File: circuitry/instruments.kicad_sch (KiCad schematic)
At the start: 70 parts, among them J38 P9-1, J39 P9-2, J40 P7-1, J41 P7-2, J42 P8-2, J43 P8-1, J49 P10-1, J50 P10-2, J53 P1-2, J54 P2-2, J55 P3-2, J56 P4-2, J57 P17-2, J58 P18-2, J59 P12-2, J60 P11-2, J63 P14-3, J64 P13-3, J72 P16-2, J73 P15-2, J76 P16-1, J77 P15-1, J78 P16-3, J79 P15-3, J81 P19-2, J82 P17-1, J83 P18-1, J88 P5-1, J89 P6-1, J90 P5-2, J91 P6-2, J92 P6-3, J93 P5-3, M1 105ZDY08, M2 12025, M3 9733, SW1 6A Momentary, SW2 6A SPDT, SW3 6A SPDT, SW4 6A Momentary SPDT, SW5 6A SPDT

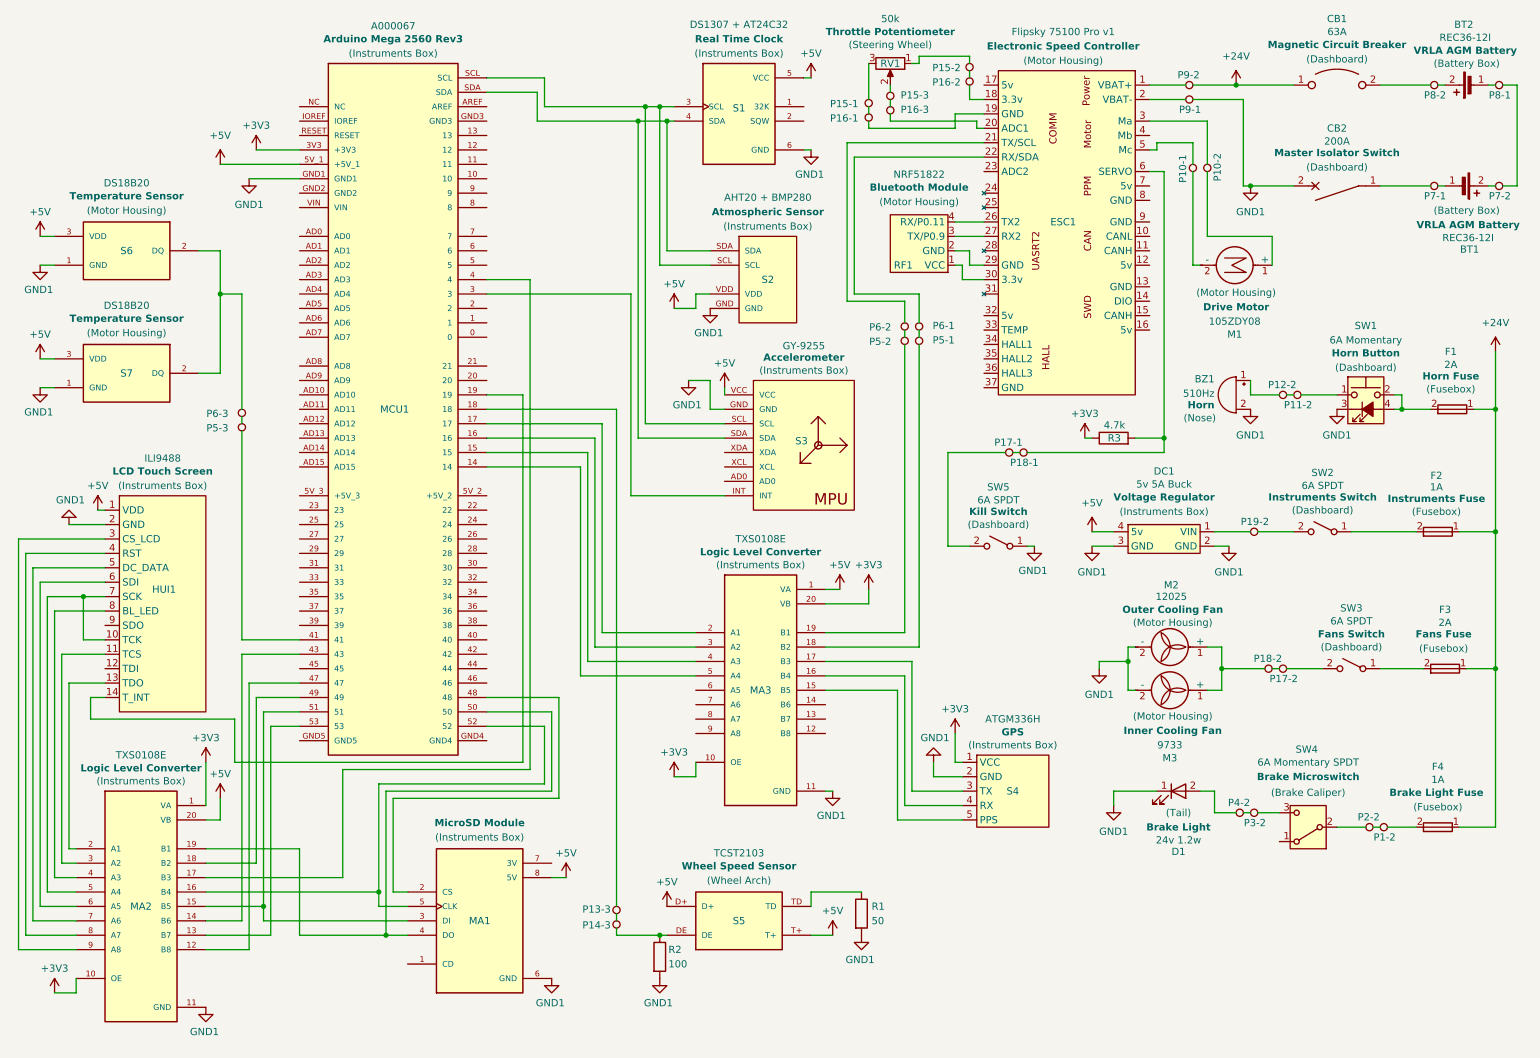
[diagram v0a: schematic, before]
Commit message: feat: Major circuit revision & refactor
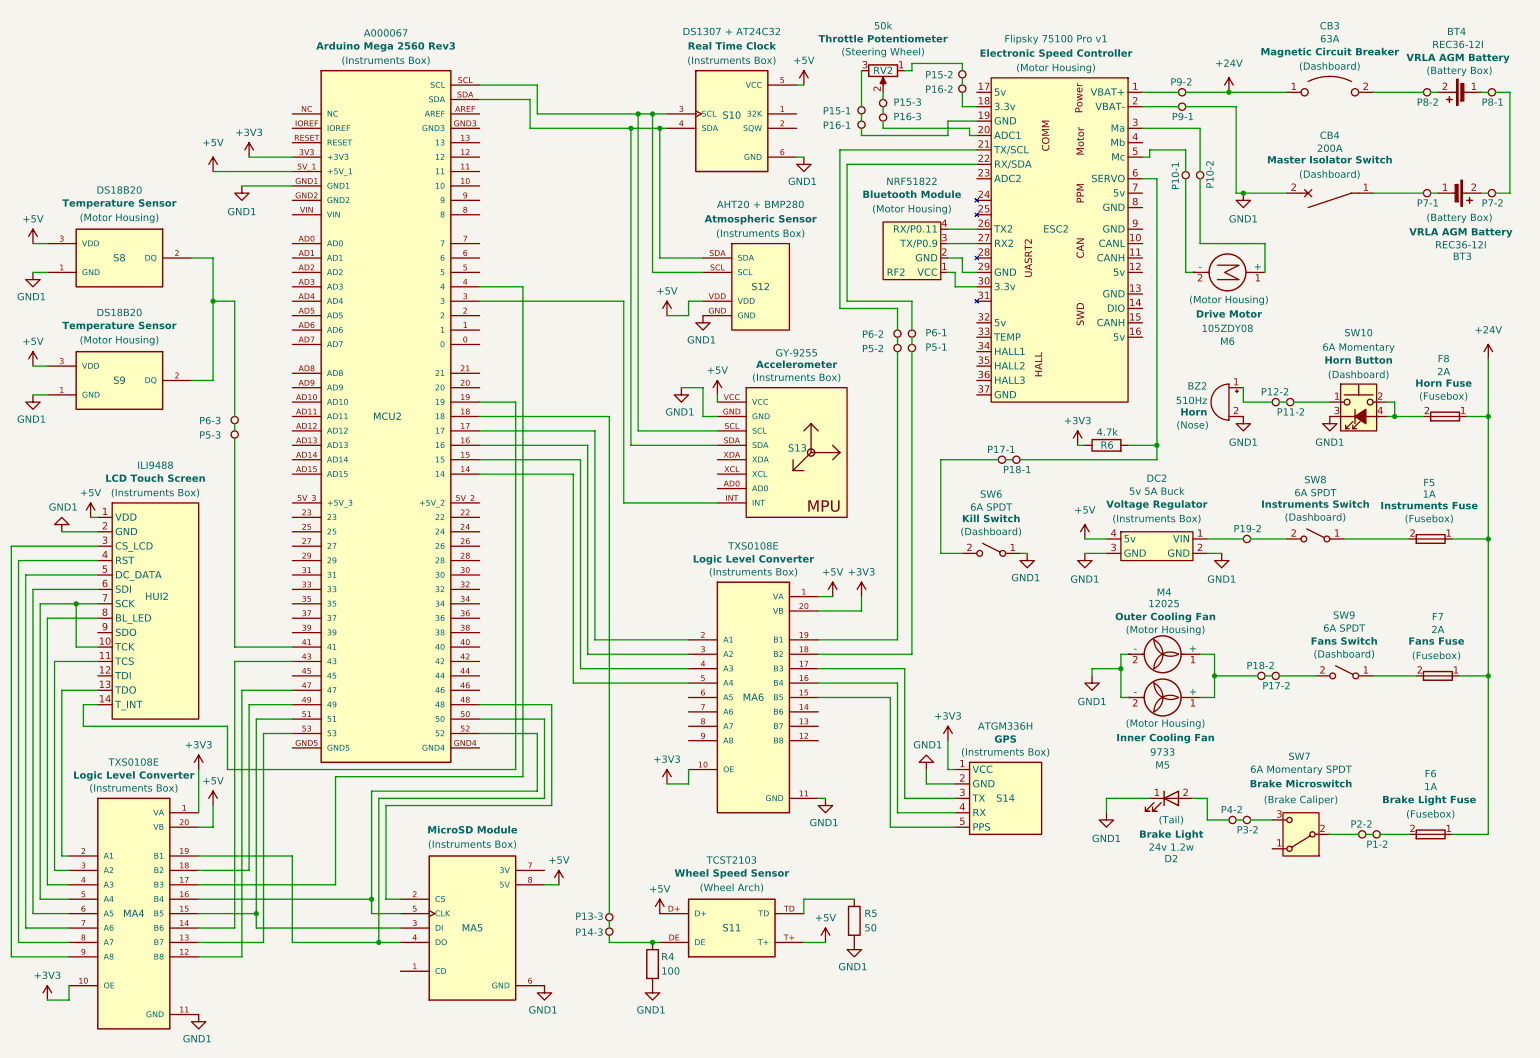
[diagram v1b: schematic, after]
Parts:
- removed BT1, BT2: REC36-12I, symbol Device:Battery_Cell
- removed BZ1: 510Hz, symbol Device:Buzzer
- removed CB1: 63A, symbol Device:CircuitBreaker_1P_US
- removed CB2: 200A, symbol Device:CircuitBreaker_1P
- removed D1: 24v 1.2w, symbol Device:LED
- removed DC1: 5v 5A Buck, symbol Custom:DC-DC
- removed ESC1: Flipsky 75100 Pro v1, symbol Custom:Flipsky_75100
- removed F1, F3: 2A, symbol Device:Fuse
- removed F2, F4: 1A, symbol Device:Fuse
- removed HUI1: ILI9488, symbol Custom:ILI9488_Display
- removed J38: P9-1, symbol Connector:TestPoint
- removed J39: P9-2, symbol Connector:TestPoint
- removed J40: P7-1, symbol Connector:TestPoint
- removed J41: P7-2, symbol Connector:TestPoint
- removed J42: P8-2, symbol Connector:TestPoint
- removed J43: P8-1, symbol Connector:TestPoint
- removed J49: P10-1, symbol Connector:TestPoint
- removed J50: P10-2, symbol Connector:TestPoint
- removed J53: P1-2, symbol Connector:TestPoint
- removed J54: P2-2, symbol Connector:TestPoint
- removed J55: P3-2, symbol Connector:TestPoint
- removed J56: P4-2, symbol Connector:TestPoint
- removed J57: P17-2, symbol Connector:TestPoint
- removed J58: P18-2, symbol Connector:TestPoint
- removed J59: P12-2, symbol Connector:TestPoint
- removed J60: P11-2, symbol Connector:TestPoint
- removed J63: P14-3, symbol Connector:TestPoint
- removed J64: P13-3, symbol Connector:TestPoint
- removed J72: P16-2, symbol Connector:TestPoint
- removed J73: P15-2, symbol Connector:TestPoint
- removed J76: P16-1, symbol Connector:TestPoint
- removed J77: P15-1, symbol Connector:TestPoint
- removed J78: P16-3, symbol Connector:TestPoint
- removed J79: P15-3, symbol Connector:TestPoint
- removed J81: P19-2, symbol Connector:TestPoint
- removed J82: P17-1, symbol Connector:TestPoint
- removed J83: P18-1, symbol Connector:TestPoint
- removed J88: P5-1, symbol Connector:TestPoint
- removed J89: P6-1, symbol Connector:TestPoint
- removed J90: P5-2, symbol Connector:TestPoint
- removed J91: P6-2, symbol Connector:TestPoint
- removed J92: P6-3, symbol Connector:TestPoint
- removed J93: P5-3, symbol Connector:TestPoint
- removed M1: 105ZDY08, symbol Motor:Motor_DC
- removed M2: 12025, symbol Motor:Fan
- removed M3: 9733, symbol Motor:Fan
- removed MA1: (no value), 254:MODULE_254, symbol Micro SD Module:254
- removed MA2, MA3: TXS0108E, ZC323900:MODULE_ZC323900, symbol Logic Level Shifter:ZC323900
- removed MCU1: A000067, A000067:MODULE_A000067, symbol Arduino Mega:A000067
- removed R1: 50, symbol Device:R
- removed R2: 100, symbol Device:R
- removed R3: 4.7k, symbol Device:R
- removed RF1: NRF51822, symbol Custom:NRF51822
- removed RV1: 50k, symbol Device:R_Potentiometer
- removed S1: DS1307 + AT24C32, TC00500:MODULE_TC00500, symbol Real Time Clock:TC00500
- removed S2: AHT20 + BMP280, AHT20_BMP280:AHT20_BMP280, symbol Temperature & Pressure:AHT20_BMP280
- removed S3: GY-9255, symbol Accelerometer:GY-521
- removed S4: ATGM336H, symbol Custom:ATGM336H
- removed S5: TCST2103, TCST2103:TCST2103, symbol Beam Break Sensor:TCST2103
- removed S6, S7: DS18B20, DS18B20_:IC_DS18B20_, symbol Temperature 1 Wire:DS18B20_
- removed SW1: 6A Momentary, symbol Switch:SW_Push_LED
- removed SW2, SW3, SW5: 6A SPDT, symbol Switch:SW_SPST
- removed SW4: 6A Momentary SPDT, symbol Switch:SW_SPDT
- added BT3, BT4: REC36-12I, symbol Device:Battery_Cell
- added BZ2: 510Hz, symbol Device:Buzzer
- added CB3: 63A, symbol Device:CircuitBreaker_1P_US
- added CB4: 200A, symbol Device:CircuitBreaker_1P
- added D2: 24v 1.2w, symbol Device:LED
- added DC2: 5v 5A Buck, symbol Custom:DC-DC
- added ESC2: Flipsky 75100 Pro v1, symbol Custom:Flipsky_75100
- added F5, F6: 1A, symbol Device:Fuse
- added F7, F8: 2A, symbol Device:Fuse
- added HUI2: ILI9488, symbol Custom:ILI9488_Display
- added J100: P6-2, symbol Connector:TestPoint
- added J101: P5-2, symbol Connector:TestPoint
- added J102: P6-1, symbol Connector:TestPoint
- added J103: P5-1, symbol Connector:TestPoint
- added J104: P15-2, symbol Connector:TestPoint
- added J105: P16-2, symbol Connector:TestPoint
- added J106: P17-1, symbol Connector:TestPoint
- added J107: P18-1, symbol Connector:TestPoint
- added J108: P9-2, symbol Connector:TestPoint
- added J109: P9-1, symbol Connector:TestPoint
- added J110: P10-1, symbol Connector:TestPoint
- added J111: P10-2, symbol Connector:TestPoint
- added J112: P4-2, symbol Connector:TestPoint
- added J113: P19-2, symbol Connector:TestPoint
- added J114: P3-2, symbol Connector:TestPoint
- added J115: P18-2, symbol Connector:TestPoint
- added J116: P12-2, symbol Connector:TestPoint
- added J117: P17-2, symbol Connector:TestPoint
- added J118: P11-2, symbol Connector:TestPoint
- added J119: P2-2, symbol Connector:TestPoint
- added J120: P1-2, symbol Connector:TestPoint
- added J121: P8-2, symbol Connector:TestPoint
- added J122: P7-1, symbol Connector:TestPoint
- added J123: P8-1, symbol Connector:TestPoint
- added J124: P7-2, symbol Connector:TestPoint
- added J86: P13-3, symbol Connector:TestPoint
- added J87: P14-3, symbol Connector:TestPoint
- added J94: P6-3, symbol Connector:TestPoint
- added J95: P5-3, symbol Connector:TestPoint
- added J96: P15-1, symbol Connector:TestPoint
- added J97: P16-1, symbol Connector:TestPoint
- added J98: P15-3, symbol Connector:TestPoint
- added J99: P16-3, symbol Connector:TestPoint
- added M4: 12025, symbol Motor:Fan
- added M5: 9733, symbol Motor:Fan
- added M6: 105ZDY08, symbol Motor:Motor_DC
- added MA4, MA6: TXS0108E, ZC323900:MODULE_ZC323900, symbol Logic Level Shifter:ZC323900
- added MA5: (no value), 254:MODULE_254, symbol Micro SD Module:254
- added MCU2: A000067, A000067:MODULE_A000067, symbol Arduino Mega:A000067
- added R4: 100, symbol Device:R
- added R5: 50, symbol Device:R
- added R6: 4.7k, symbol Device:R
- added RF2: NRF51822, symbol Custom:NRF51822
- added RV2: 50k, symbol Device:R_Potentiometer
- added S10: DS1307 + AT24C32, TC00500:MODULE_TC00500, symbol Real Time Clock:TC00500
- added S11: TCST2103, TCST2103:TCST2103, symbol Beam Break Sensor:TCST2103
- added S12: AHT20 + BMP280, AHT20_BMP280:AHT20_BMP280, symbol Temperature & Pressure:AHT20_BMP280
- added S13: GY-9255, symbol Accelerometer:GY-521
- added S14: ATGM336H, symbol Custom:ATGM336H
- added S8, S9: DS18B20, DS18B20_:IC_DS18B20_, symbol Temperature 1 Wire:DS18B20_
- added SW10: 6A Momentary, symbol Switch:SW_Push_LED
- added SW6, SW8, SW9: 6A SPDT, symbol Switch:SW_SPST
- added SW7: 6A Momentary SPDT, symbol Switch:SW_SPDT
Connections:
- net +24V: now also CB3.1, F5.1, F6.1, F7.1, F8.1, J108.2
- net +3V3: now also MA4.1 (VA), MA4.10 (OE), MA6.10 (OE), MA6.20 (VB), MCU2.3V3 (+3V3), R6.1, S14.1 (VCC)
- net +5V: now also DC2.4 (5v), HUI2.1 (VDD), MA4.20 (VB), MA5.8 (5V), MA6.1 (VA), MCU2.5V_1 (+5V_1), S10.5 (VCC), S11.D+, S11.T+, S12.VDD, S13.VCC, S8.3 (VDD), S9.3 (VDD)
- net GND1: now also BZ2.2 (-), CB4.2, D2.1 (K), DC2.2 (GND), DC2.3 (GND), HUI2.2 (GND), J109.1, M4.2 (-), M5.2 (-), MA4.11 (GND), MA5.6 (GND), MA6.11 (GND), MCU2.GND1, R4.2, R5.2, S10.6 (GND), S12.GND, S13.GND, S14.2 (GND), S8.1 (GND), S9.1 (GND), SW10.3 (K), SW6.1 (A)
- new net: J87.1, R4.1, S11.DE
- new net: J94.1, S8.2 (DQ), S9.2 (DQ)
- new net: BT4.2 (+), J121.1
- new net: CB3.2, J121.2
- new net: J103.1, MA6.18 (B2)
- new net: J102.2, J103.2
- new net: MCU2.SCL, S10.3 (SCL), S12.SCL, S13.SCL
- new net: MCU2.SDA, S10.4 (SDA), S12.SDA, S13.SDA
- new net: J106.1, SW6.2 (B)
- new net: J106.2, J107.2
- new net: J123.1, J124.1
- new net: BT4.1 (-), J123.2
- new net: J111.2, M6.1 (+)
- new net: J110.1, M6.2 (-)
- new net: BZ2.1 (+), J116.1
- new net: J116.2, J118.2
- new net: F7.2, SW9.1 (A)
- new net: J86.2, J87.2
- new net: ESC2.6 (SERVO), J107.1, R6.2
- new net: BT3.2 (+), J124.2
- new net: D2.2 (A), J112.1
- new net: F6.2, J120.1
- new net: CB4.1, J122.2
- new net: J94.2, J95.2
- new net: J119.2, J120.2
- new net: J104.1, RV2.1
- new net: J104.2, J105.2
- new net: ESC2.19 (GND), J97.1
- new net: J96.2, J97.2
- new net: ESC2.22 (RX/SDA), J102.1
- new net: J86.1, MCU2.18
- new net: J118.1, SW10.1
- new net: J98.1, RV2.2
- new net: J96.1, RV2.3
- new net: MA5.2 (CS), MCU2.48
- new net: MA4.15 (B5), MA5.3 (DI), MCU2.51
- new net: MA4.19 (B1), MA5.4 (DO), MCU2.50
- new net: MA4.16 (B4), MA5.5 (CLK), MCU2.52
- new net: ESC2.1 (VBAT+), J108.1
- new net: ESC2.18 (3.3v), J105.1
- new net: ESC2.2 (VBAT-), J109.2
- new net: ESC2.20 (ADC1), J99.1
- new net: ESC2.21 (TX/SCL), J100.1
- new net: ESC2.26 (TX2), RF2.4 (RX/P0.11)
- new net: ESC2.27 (RX2), RF2.3 (TX/P0.9)
- new net: ESC2.29 (GND), RF2.2 (GND)
- new net: ESC2.3 (Ma), J111.1
- new net: ESC2.30 (3.3v), RF2.1 (VCC)
- new net: ESC2.5 (Mc), J110.2
- new net: J113.1, SW8.2 (B)
- new net: DC2.1 (VIN), J113.2
- new net: J114.1, SW7.3 (C)
- new net: J112.2, J114.2
- new net: J119.1, SW7.2 (B)
- new net: MA6.17 (B3), S14.3 (TX)
- new net: MA6.16 (B4), S14.4 (RX)
- new net: MA6.15 (B5), S14.5 (PPS)
- new net: J95.1, MCU2.41
- new net: F8.2, SW10.2, SW10.4 (A)
- new net: J98.2, J99.2
- new net: BT3.1 (-), J122.1
- new net: J115.1, M4.1 (+), M5.1 (+)
- new net: J115.2, J117.2
- new net: R5.1, S11.TD
- new net: F5.2, SW8.1 (A)
- new net: MA4.12 (B8), MCU2.47
- new net: MA4.13 (B7), MCU2.53
- new net: MA4.14 (B6), MCU2.43
- new net: MA4.17 (B3), MCU2.4
- new net: MA4.18 (B2), MCU2.49
- new net: HUI2.13 (TDO), MA4.2 (A1)
- new net: HUI2.11 (TCS), MA4.3 (A2)
- new net: HUI2.8 (BL_LED), MA4.4 (A3)
- new net: HUI2.10 (TCK), HUI2.7 (SCK), MA4.5 (A4)
- new net: HUI2.6 (SDI), MA4.6 (A5)
- new net: HUI2.5 (DC_DATA), MA4.7 (A6)
- new net: HUI2.4 (RST), MA4.8 (A7)
- new net: HUI2.3 (CS_LCD), MA4.9 (A8)
- new net: J117.1, SW9.2 (B)
- new net: J101.1, MA6.19 (B1)
- new net: MA6.2 (A1), MCU2.17
- new net: MA6.3 (A2), MCU2.16
- new net: MA6.4 (A3), MCU2.15
- new net: MA6.5 (A4), MCU2.14
- new net: J100.2, J101.2
- new net: MCU2.3, S13.INT
- new net: HUI2.14 (T_INT), MCU2.19
